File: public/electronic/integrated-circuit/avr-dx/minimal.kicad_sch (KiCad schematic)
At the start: 12 parts, among them P1 USB_C_Plug_USB2.0, U1 AVR128DA48x-xPT, U2 CH340C

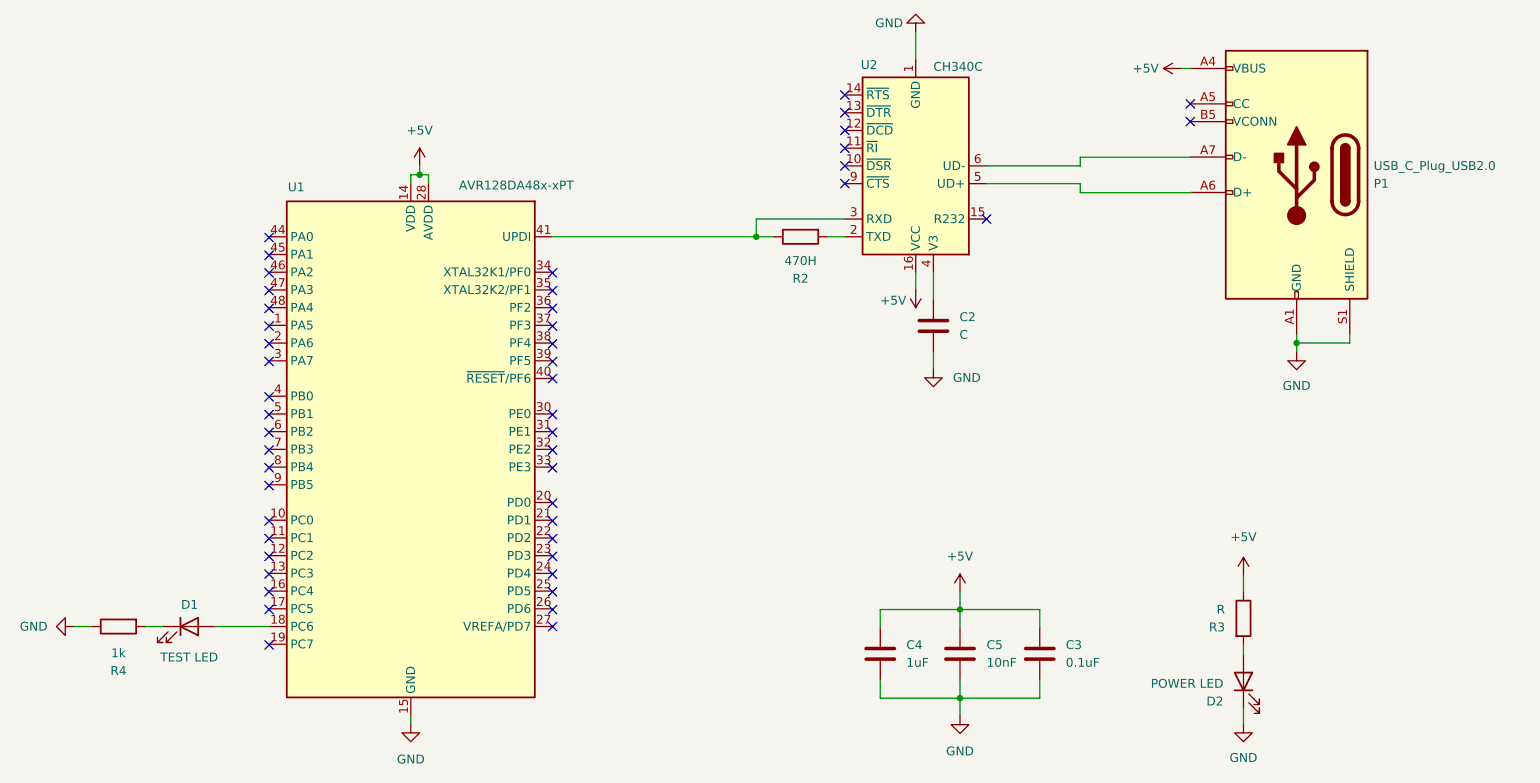
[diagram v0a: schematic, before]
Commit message: Save changes at: 1753983998
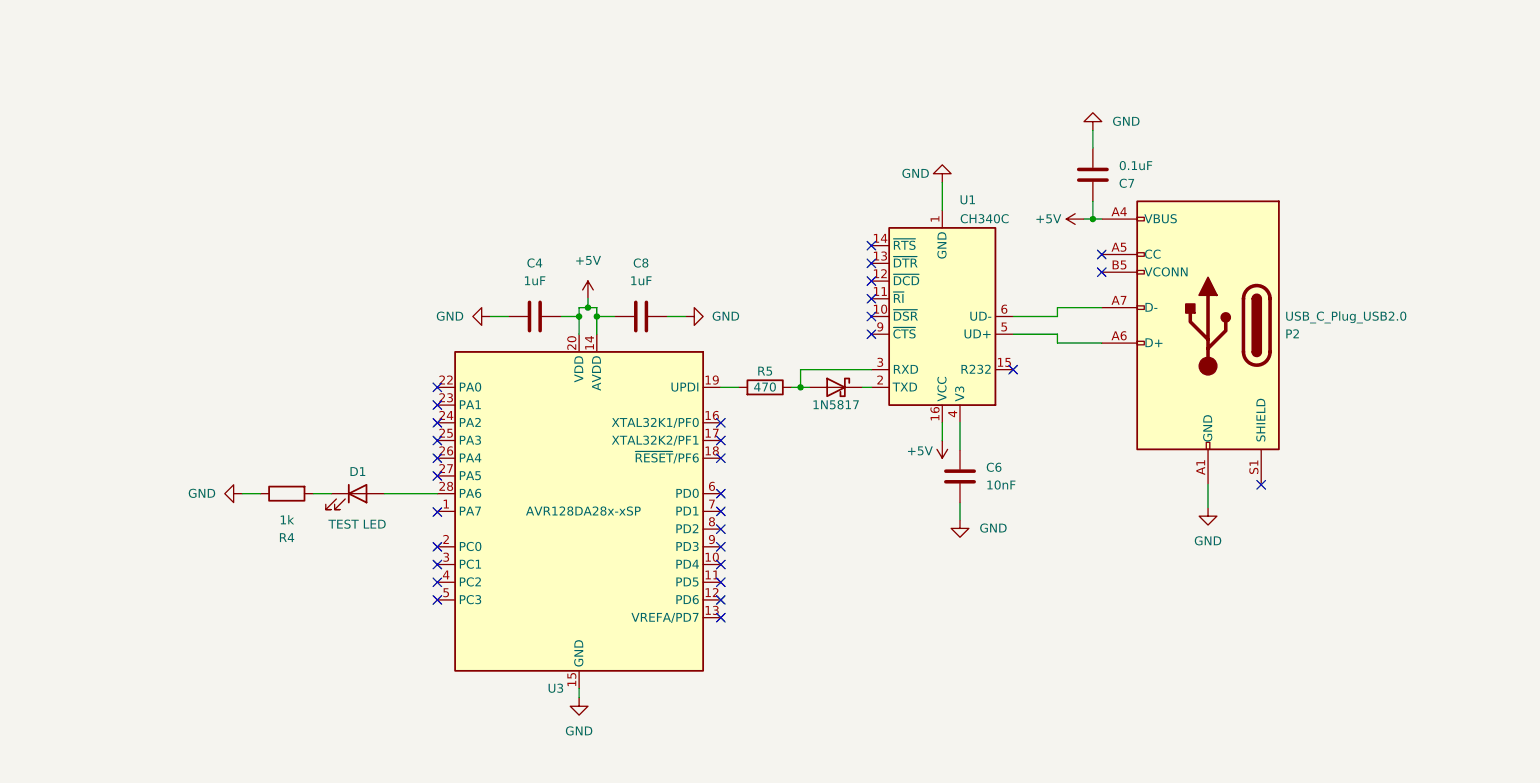
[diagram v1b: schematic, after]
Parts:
- removed C2: C, symbol Device:C
- removed C3: 0.1uF, symbol Device:C
- removed C5: 10nF, symbol Device:C
- removed D2: POWER LED, symbol Device:LED
- removed P1: USB_C_Plug_USB2.0, symbol Connector:USB_C_Plug_USB2.0
- removed R3: R, symbol Device:R
- removed U1: AVR128DA48x-xPT, Package_QFP:TQFP-48_7x7mm_P0.5mm, symbol MCU_Microchip_AVR_Dx:AVR128DA48x-xPT
- removed U2: CH340C, Package_SO:SOIC-16_3.9x9.9mm_P1.27mm, symbol Interface_USB:CH340C
- added C6: 10nF, symbol Device:C
- added C7: 0.1uF, symbol Device:C
- added C8: 1uF, symbol Device:C
- added D3: 1N5817, Diode_THT:D_DO-41_SOD81_P10.16mm_Horizontal, symbol Diode:1N5817
- added P2: USB_C_Plug_USB2.0, symbol Connector:USB_C_Plug_USB2.0
- added U1: CH340C, Package_SO:SOIC-16_3.9x9.9mm_P1.27mm, symbol Interface_USB:CH340C
- added U3: AVR128DA28x-xSP, Package_DIP:DIP-28_W7.62mm, symbol MCU_Microchip_AVR_Dx:AVR128DA28x-xSP
- R5: renamed from R2; value 470H -> 470; footprint (none) -> Resistor_SMD:R_1206_3216Metric_Pad1.30x1.75mm_HandSolder
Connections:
- net +5V: now also C4.1, C7.2, C8.2, P2.A4 (VBUS), P2.A9 (VBUS), P2.B4 (VBUS), P2.B9 (VBUS), U1.16 (VCC), U3.14 (AVDD), U3.20 (VDD); no longer C4.2
- net GND: now also C4.2, C6.1, C7.1, C8.1, P2.A1 (GND), P2.A12 (GND), P2.B1 (GND), P2.B12 (GND), U1.1 (GND), U3.15 (GND), U3.21 (GND); no longer C4.1
- net at D1.2 (A): now also U3.28 (PA6)
- net at R5.1: now also D3.2 (A), U1.3 (RXD)
- net at R5.2: now also U3.19 (UPDI)
- new net: D3.1 (K), U1.2 (TXD)
- new net: C6.2, U1.4 (V3)
- new net: P2.A6 (D+), U1.5 (UD+)
- new net: P2.A7 (D-), U1.6 (UD-)
- no-connect marks 49 -> 32
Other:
- moved on the sheet: C4, D1, R4, R5
